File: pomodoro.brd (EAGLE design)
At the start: 33.6 x 33.6 mm, 11 parts, among them IC1 ATTINY13V-10PU, SW1 1825910-6

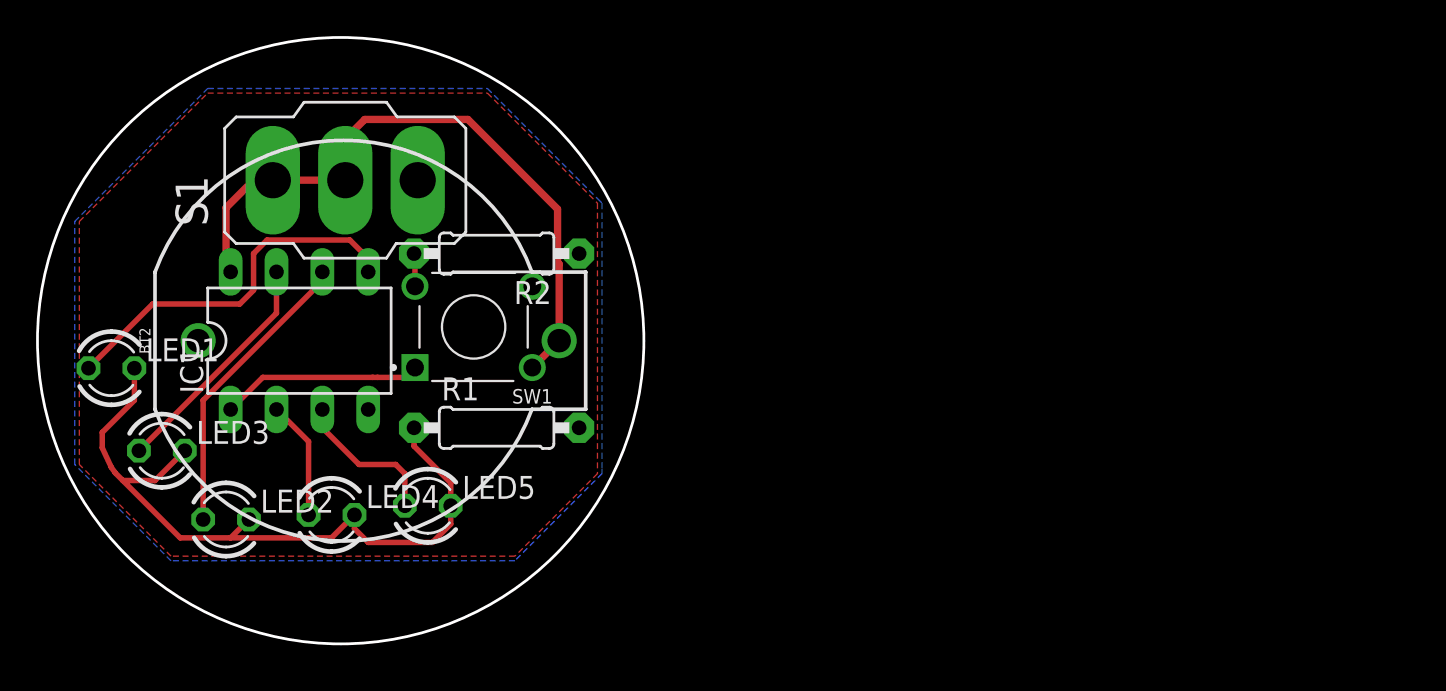
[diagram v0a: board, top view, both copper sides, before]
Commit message: curcuit changed
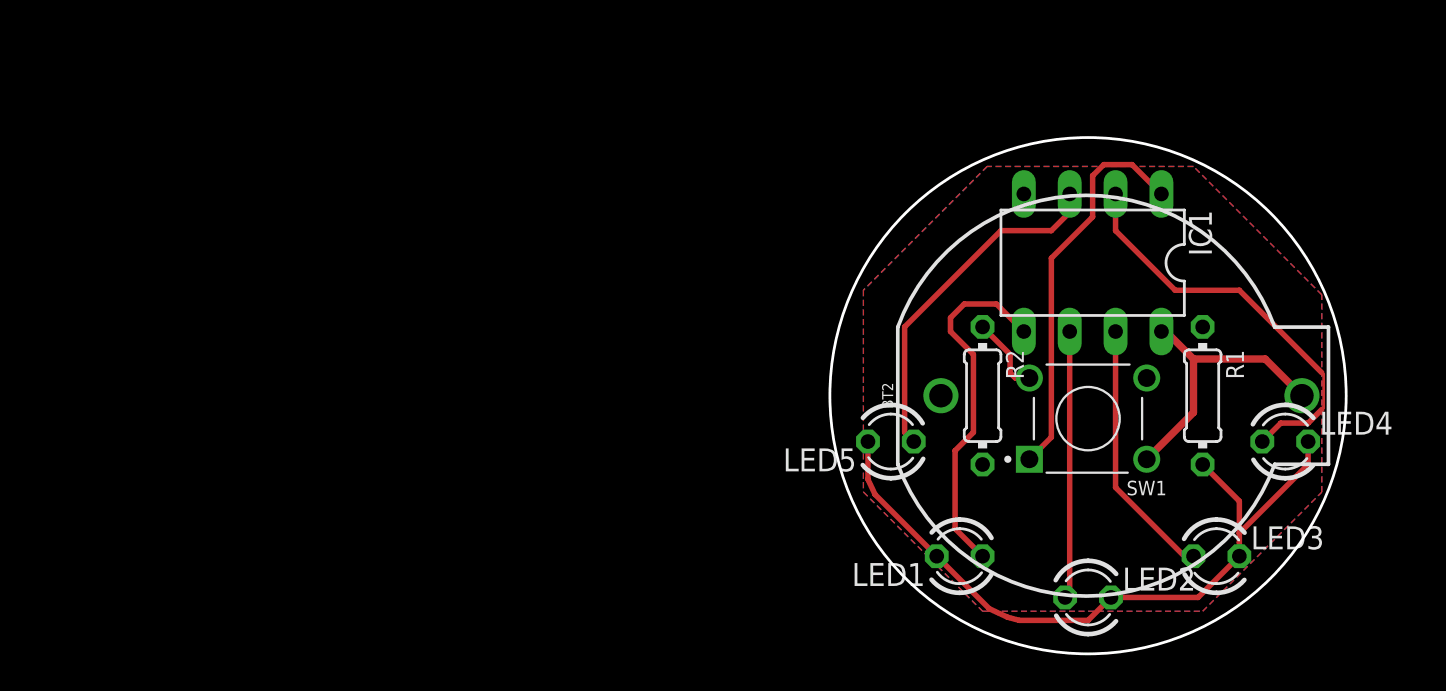
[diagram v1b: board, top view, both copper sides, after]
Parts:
- removed S1: (no value), switch:320-916
- R1, R2: device adafruit:0207/9 -> rcl:0204/7
- moved LED3 58.7 mm to (62.2, 7.11)
- moved LED4 53.0 mm to (66.0, 13.5)
- moved LED1 48.1 mm to (48.0, 7.11), turned to 180 degrees
- moved LED2 47.9 mm to (55.1, 4.83)
- moved IC1 44.2 mm to (55.4, 23.4), turned to 180 degrees
- moved BT2 41.3 mm to (55.1, 16.0)
- moved R1 39.2 mm to (61.5, 16.0), turned to 270 degrees
- moved SW1 34.4 mm to (55.1, 14.7)
- moved R2 28.1 mm to (49.3, 16.0), turned to 270 degrees
- moved LED5 25.9 mm to (44.2, 13.5), turned to 180 degrees
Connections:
- net GND: now also R1.1, R2.2; no longer R1.2, R2.1, S1.3
- net N$6: now also R1.2; no longer R1.1
- net N$8: now also R2.1; no longer R2.2
- net VCC: no longer S1.1, S1.2
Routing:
- net VCC: track 36.9 -> 15.9 mm
- net N$4: track 6.58 -> 22.9 mm
- net N$7: track 11.2 -> 22.4 mm
- net N$5: track 8.42 -> 19.4 mm
- net N$8: track 1.84 -> 4.36 mm
- net N$2: track 16.5 -> 14.8 mm
- net N$3: track 13.1 -> 14.5 mm
- net N$1: track 20.8 -> 19.8 mm
- net N$6: track 40.5 -> 40.0 mm
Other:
- board size 33.6 x 33.6 mm -> 28.6 x 28.6 mm
